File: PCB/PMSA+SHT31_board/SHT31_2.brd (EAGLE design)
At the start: 41.7 x 49.2 mm, 18 parts, among them CN2 CON_PINHD-2X15, Q3 MOSFET-NCHANNELBSS138, U2 SHT31-DIS, U3 MICS-4514

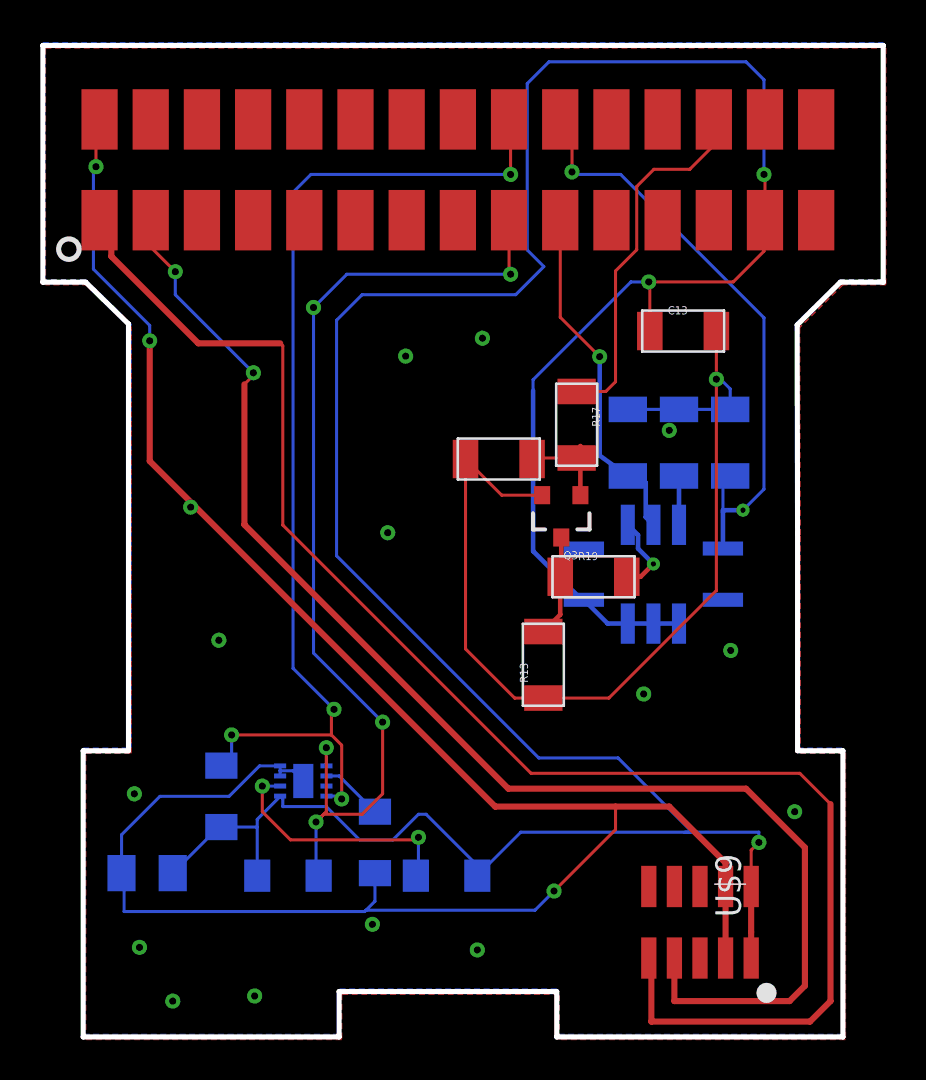
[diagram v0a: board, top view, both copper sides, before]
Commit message: 3DPACKAGE!
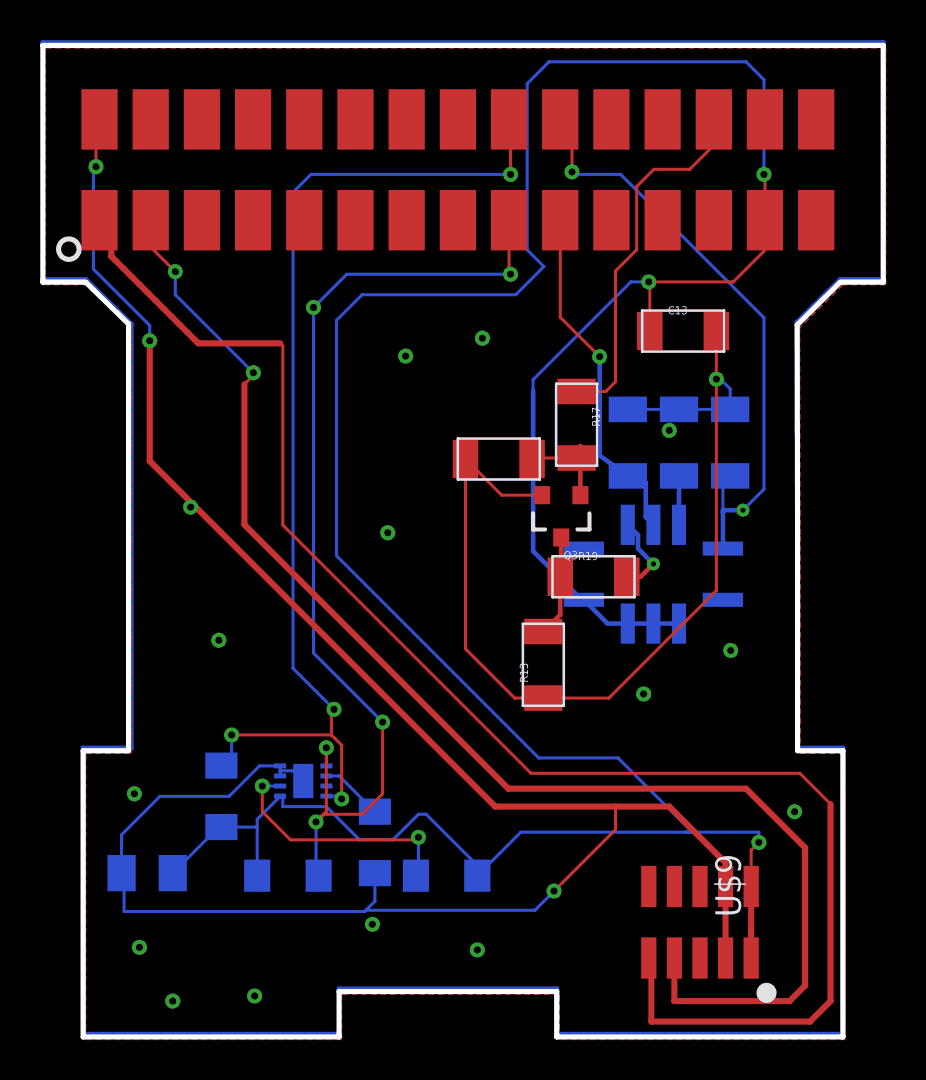
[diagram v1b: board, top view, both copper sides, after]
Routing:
- net GND: track 154.2 -> 347.2 mm
